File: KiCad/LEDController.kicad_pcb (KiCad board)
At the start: 4 copper layers, 50 x 50 mm, 40 parts, among them J1 Conn_01x05, J2 UART, J3 JTAG, J5 USB_C_Receptacle_USB2.0_16P, J6 Conn_01x03, J7 VDD, J8 GND, J9 Conn_01x14, Q1 IRLZ44N, Q2 IRLZ44N, Q3 IRLZ44N, Q4 IRLZ44N, SW1 BOOT, SW2 ENABLE, U1 TPS62132, U2 ESP32-S3-WROOM-2

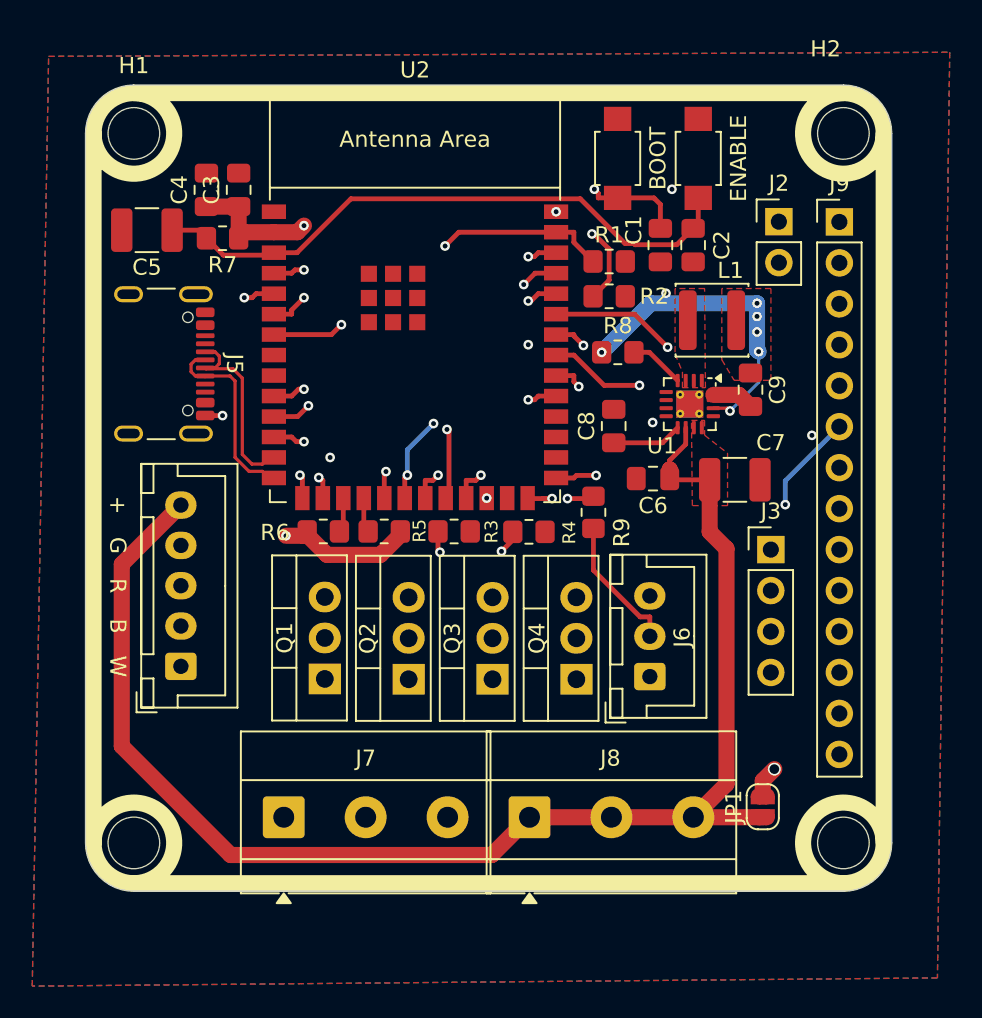
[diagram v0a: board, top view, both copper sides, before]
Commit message: rearrange again, route
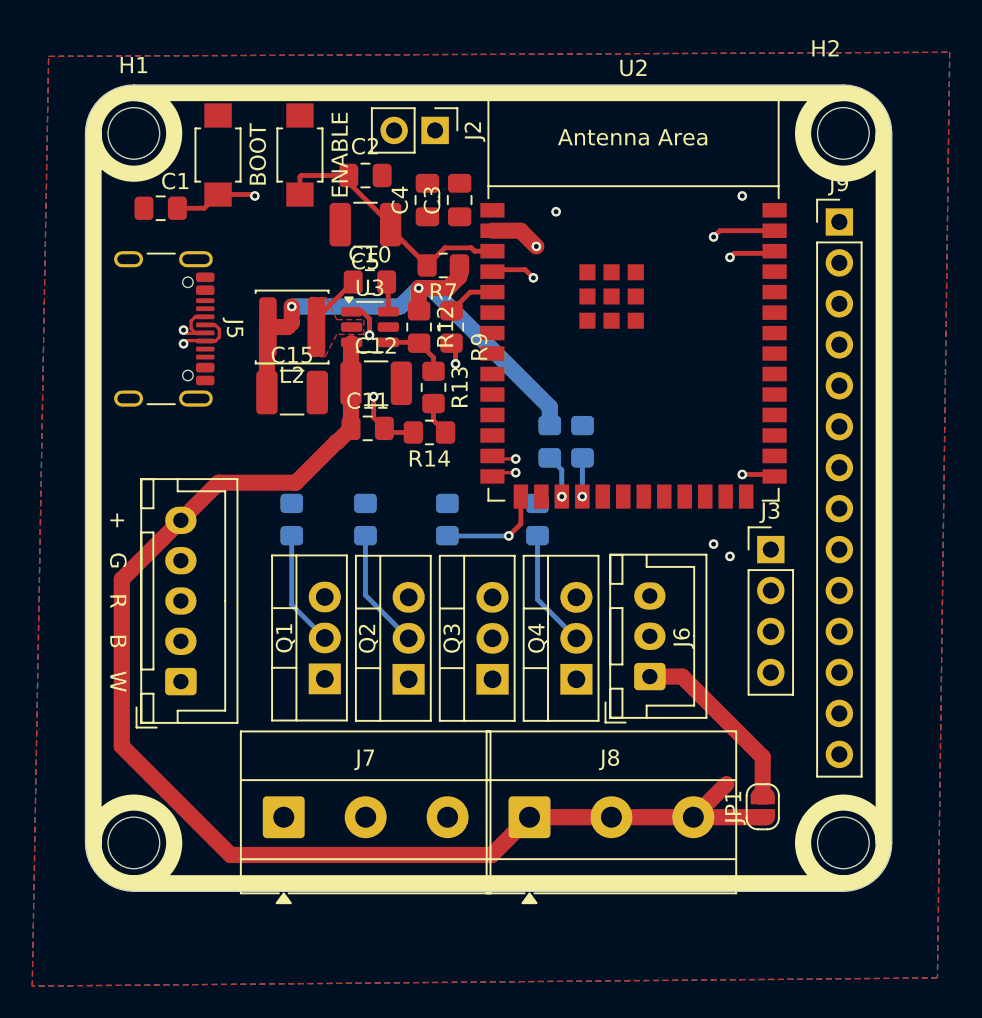
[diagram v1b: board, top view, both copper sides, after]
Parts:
- removed C6: 100n, Capacitor_SMD:C_0805_2012Metric_Pad1.18x1.45mm_HandSolder
- removed C7: 10u, Capacitor_SMD:C_1210_3225Metric_Pad1.33x2.70mm_HandSolder
- removed C8: 3.3n, Capacitor_SMD:C_0805_2012Metric_Pad1.18x1.45mm_HandSolder
- removed C9: 22u, Capacitor_SMD:C_0805_2012Metric_Pad1.18x1.45mm_HandSolder
- removed L1: 1/2.2u, Inductor_SMD:L_APV_ANR4026
- removed R8: 100k, Resistor_SMD:R_0805_2012Metric_Pad1.20x1.40mm_HandSolder
- removed U1: TPS62132, Package_DFN_QFN:VQFN-16-1EP_3x3mm_P0.5mm_EP1.68x1.68mm_ThermalVias
- added C10: 100n, Capacitor_SMD:C_0805_2012Metric_Pad1.18x1.45mm_HandSolder, F.Cu at (102.6, 61.2)
- added C11: 100n, Capacitor_SMD:C_0805_2012Metric_Pad1.18x1.45mm_HandSolder, F.Cu at (102.5, 70.3)
- added C12: 10u, Capacitor_SMD:C_1210_3225Metric_Pad1.33x2.70mm_HandSolder, F.Cu at (103.0, 67.5)
- added C15: 10u, Capacitor_SMD:C_1210_3225Metric_Pad1.33x2.70mm_HandSolder, F.Cu at (97.8, 68.1)
- added L2: 15u, Inductor_SMD:L_APV_ANR4026, F.Cu at (97.8, 64.0)
- added R12: 100k, Resistor_SMD:R_0805_2012Metric_Pad1.20x1.40mm_HandSolder, F.Cu at (105.7, 64.0)
- added R13: 1.8k, Resistor_SMD:R_0805_2012Metric_Pad1.20x1.40mm_HandSolder, F.Cu at (106.6, 67.8)
- added R14: 20k, Resistor_SMD:R_0805_2012Metric_Pad1.20x1.40mm_HandSolder, F.Cu at (106.3, 70.5)
- added U3: TPS54202DDC, Package_TO_SOT_SMD:SOT-23-6, F.Cu at (102.6, 64.0)
- R1, R2, R3, R4, R5, R6: moved to B.Cu
- moved C1 31.1 mm to (89.7, 56.6), turned to 0 degrees
- moved R1 25.4 mm to (97.8, 75.9), turned to 90 degrees
- moved SW1 24.8 mm to (93.2, 53.3)
- moved SW2 24.7 mm to (98.3, 53.3)
- moved J2 22.1 mm to (106.7, 51.8), turned to -90 degrees
- moved C2 20.8 mm to (102.4, 54.6), turned to 180 degrees
- moved R2 20.5 mm to (102.4, 75.9), turned to 90 degrees
- moved R6 15.1 mm to (113.8, 71.1), turned to -90 degrees
- moved R9 14.5 mm to (107.7, 64.0)
- moved R7 13.8 mm to (107.2, 60.2)
- moved C3 13.7 mm to (108.2, 56.1)
- moved C4 13.7 mm to (106.2, 56.1)
- moved C5 13.6 mm to (102.4, 57.7)
- moved U2 13.6 mm to (119.0, 65.0)
- moved R5 13.5 mm to (115.8, 71.1), turned to -90 degrees
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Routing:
- net GPIO.6: track 47.3 -> 0.00 mm, vias 1 -> 0
- net +3.3V: track 89.4 -> 43.9 mm, vias 10 -> 3
- net GPIO.11: track 45.4 -> 0.00 mm, vias 1 -> 0
- net GPIO.8: track 42.9 -> 0.00 mm, vias 1 -> 0
- net GPIO.18: track 40.0 -> 0.00 mm, vias 1 -> 0
- net GPIO.46: track 39.8 -> 0.00 mm, vias 1 -> 0
- net GPIO.17: track 39.0 -> 0.00 mm, vias 1 -> 0
- net GPIO.7: track 36.9 -> 0.00 mm, vias 1 -> 0
- net GPIO.38: track 35.5 -> 0.00 mm, vias 2 -> 0
- net GPIO.12: track 33.8 -> 0.00 mm, vias 2 -> 0
- net GPIO.47: track 32.6 -> 0.00 mm, vias 1 -> 0
- net JTAG.MTMS: track 31.9 -> 0.00 mm, vias 1 -> 0
- net GPIO.13: track 31.1 -> 0.00 mm, vias 2 -> 0
- net GPIO.45: track 30.2 -> 0.00 mm, vias 1 -> 0
- net GPIO.14: track 30.1 -> 0.00 mm, vias 1 -> 0
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- added copper zone on F.Cu, net Net-(U3-SW)
- removed copper zone on F.Cu, net +24V
- removed copper zone on F.Cu, net +3.3V
- removed copper zone on F.Cu, net /3.3V Switch
